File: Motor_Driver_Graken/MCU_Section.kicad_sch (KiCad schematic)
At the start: 35 parts, among them U5 STM32F405RGTx, U8 74LVC1G04, Y1 Crystal

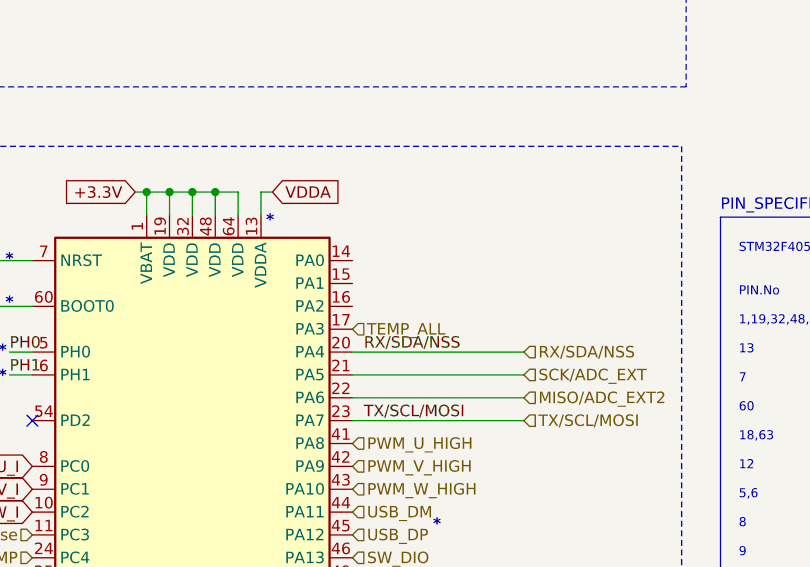
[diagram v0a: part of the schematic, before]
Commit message: Schematic Changes
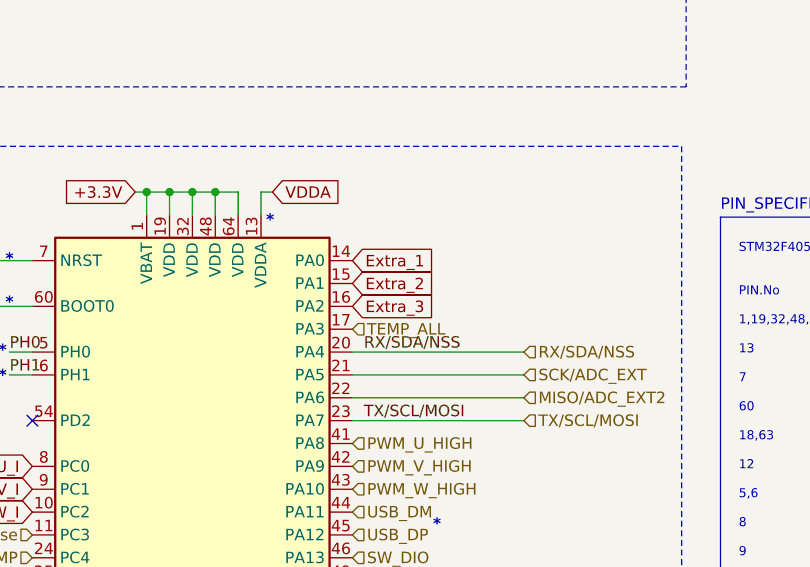
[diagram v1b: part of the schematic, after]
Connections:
- net Extra_1: now reaches U5.14 (PA0)
- net Extra_2: now reaches U5.15 (PA1)
- net Extra_3: now reaches U5.16 (PA2)
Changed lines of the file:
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@@
+		)
+	)
+	(global_label "Extra_3"
+		(shape input)
+		(at 100.33 95.25 0)
+		(fields_autoplaced yes)
+		(effects
+			(font
+				(size 1.27 1.27)
+			)
+			(justify left)
+		)
+		(property "Intersheetrefs" "${INTERSHEET_REFS}"
+			(at 110.3303 95.25 0)
+			(effects
+				(font
+					(size 1.27 1.27)
+				)
+				(justify left)
+				(hide yes)
+			)
 		)
 	)
@@
 				(hide yes)
 			)
+		)
+	)
+	(global_label "Extra_1"
+		(shape input)
+		(at 100.33 90.17 0)
+		(fields_autoplaced yes)
+		(effects
+			(font
+				(size 1.27 1.27)
+			)
+			(justify left)
+		)
+		(property "Intersheetrefs" "${INTERSHEET_REFS}"
+			(at 110.3303 90.17 0)
+			(effects
+				(font
+					(size 1.27 1.27)
+				)
+				(justify left)
+				(hide yes)
+			)
+		)
+	)
+	(global_label "Extra_2"
+		(shape input)
+		(at 100.33 92.71 0)
+		(fields_autoplaced yes)
+		(effects
+			(font
+				(size 1.27 1.27)
+			)
+			(justify left)
+		)
+		(property "Intersheetrefs" "${INTERSHEET_REFS}"
+			(at 110.3303 92.71 0)
+			(effects
+				(font
+					(size 1.27 1.27)
+				)
+				(justify left)
+				(hide yes)
+			)
